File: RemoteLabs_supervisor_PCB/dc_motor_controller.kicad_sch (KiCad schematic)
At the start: 7 parts, among them J16 MotorController_PWR_IP, J17 MotorController_PWR_OP, J18 Motor Output

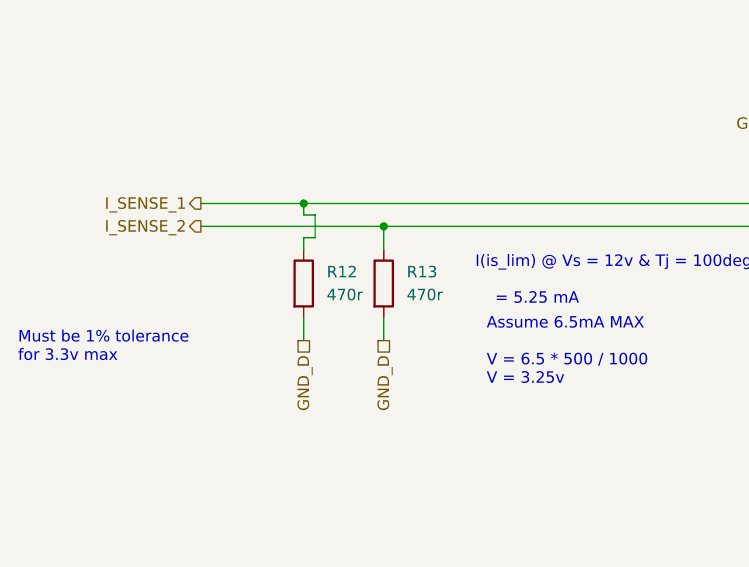
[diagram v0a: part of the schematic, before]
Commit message: mbncmvbc,
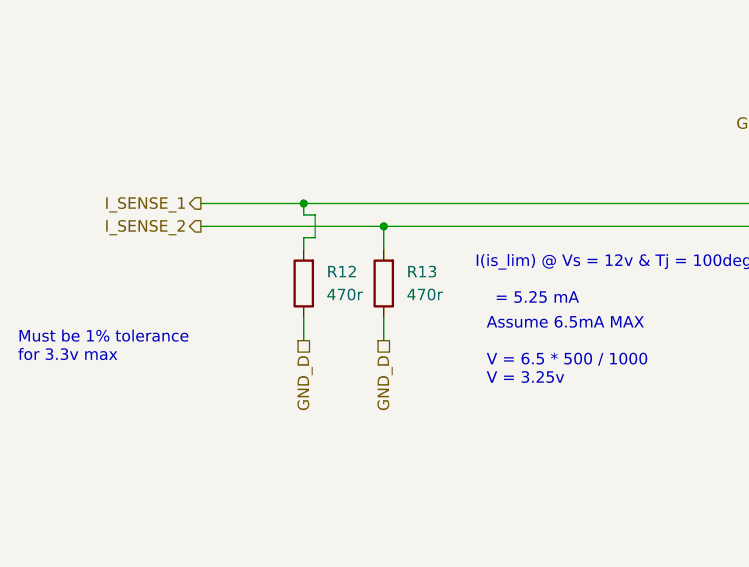
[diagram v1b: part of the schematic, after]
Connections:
- net GND_D: now also R12.1, R13.1; no longer R12.2, R13.2
- net I_SENSE_1: now also R12.2; no longer R12.1
- net I_SENSE_2: now also R13.2; no longer R13.1
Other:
- moved on the sheet: R12, R13
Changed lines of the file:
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@@
     (pin "9")
   )
-  (symbol (lib_id "000_Resistors_Immo:Resistor_0805") (at 63.5 118.11 0) (unit 1)
+  (symbol (lib_id "000_Resistors_Immo:Resistor_0805") (at 63.5 118.11 90) (unit 1)
     (in_bom yes) (on_board yes) (fields_autoplaced)
-    (property "Reference" "R12" (id 0) (at 66.04 116.8399 0)
-      (effects (font (size 1.27 1.27)) (justify left))
+    (property "Reference" "R12" (id 0) (at 66.04 116.8399 90)
+      (effects (font (size 1.27 1.27)) (justify right))
     )
-    (property "Value" "470r" (id 1) (at 66.04 119.3799 0)
-      (effects (font (size 1.27 1.27)) (justify left))
+    (property "Value" "470r" (id 1) (at 66.04 119.3799 90)
+      (effects (font (size 1.27 1.27)) (justify right))
     )
-    (property "Footprint" "Resistor_SMD:R_0805_2012Metric_Pad1.20x1.40mm_HandSolder" (id 2) (at 61.722 118.11 90)
+    (property "Footprint" "Resistor_SMD:R_0805_2012Metric_Pad1.20x1.40mm_HandSolder" (id 2) (at 63.5 119.888 90)
       (effects (font (size 1.27 1.27)) hide)
     )
@@
     (pin "3")
   )
-  (symbol (lib_id "000_Resistors_Immo:Resistor_0805") (at 72.39 118.11 0) (unit 1)
+  (symbol (lib_id "000_Resistors_Immo:Resistor_0805") (at 72.39 118.11 90) (unit 1)
     (in_bom yes) (on_board yes) (fields_autoplaced)
-    (property "Reference" "R13" (id 0) (at 74.93 116.8399 0)
-      (effects (font (size 1.27 1.27)) (justify left))
+    (property "Reference" "R13" (id 0) (at 74.93 116.8399 90)
+      (effects (font (size 1.27 1.27)) (justify right))
     )
-    (property "Value" "470r" (id 1) (at 74.93 119.3799 0)
-      (effects (font (size 1.27 1.27)) (justify left))
+    (property "Value" "470r" (id 1) (at 74.93 119.3799 90)
+      (effects (font (size 1.27 1.27)) (justify right))
     )
-    (property "Footprint" "Resistor_SMD:R_0805_2012Metric_Pad1.20x1.40mm_HandSolder" (id 2) (at 70.612 118.11 90)
+    (property "Footprint" "Resistor_SMD:R_0805_2012Metric_Pad1.20x1.40mm_HandSolder" (id 2) (at 72.39 119.888 90)
       (effects (font (size 1.27 1.27)) hide)
     )
@@
     (pin "2")
   )
-  (symbol (lib_name "Screw_Terminal_01x03_1") (lib_id "Connector:Screw_Terminal_01x03") (at 144.78 156.21 270) (unit 1)
+  (symbol (lib_id "Connector:Screw_Terminal_01x03") (at 144.78 156.21 270) (unit 1)
     (in_bom yes) (on_board yes)
     (property "Reference" "J18" (id 0) (at 149.86 154.9399 90)
